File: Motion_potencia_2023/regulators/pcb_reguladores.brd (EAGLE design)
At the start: 200 x 95 mm, 19 parts, among them P1 USB-A1HSW6, X1 5566-25569-2, X3 5566-25569-2

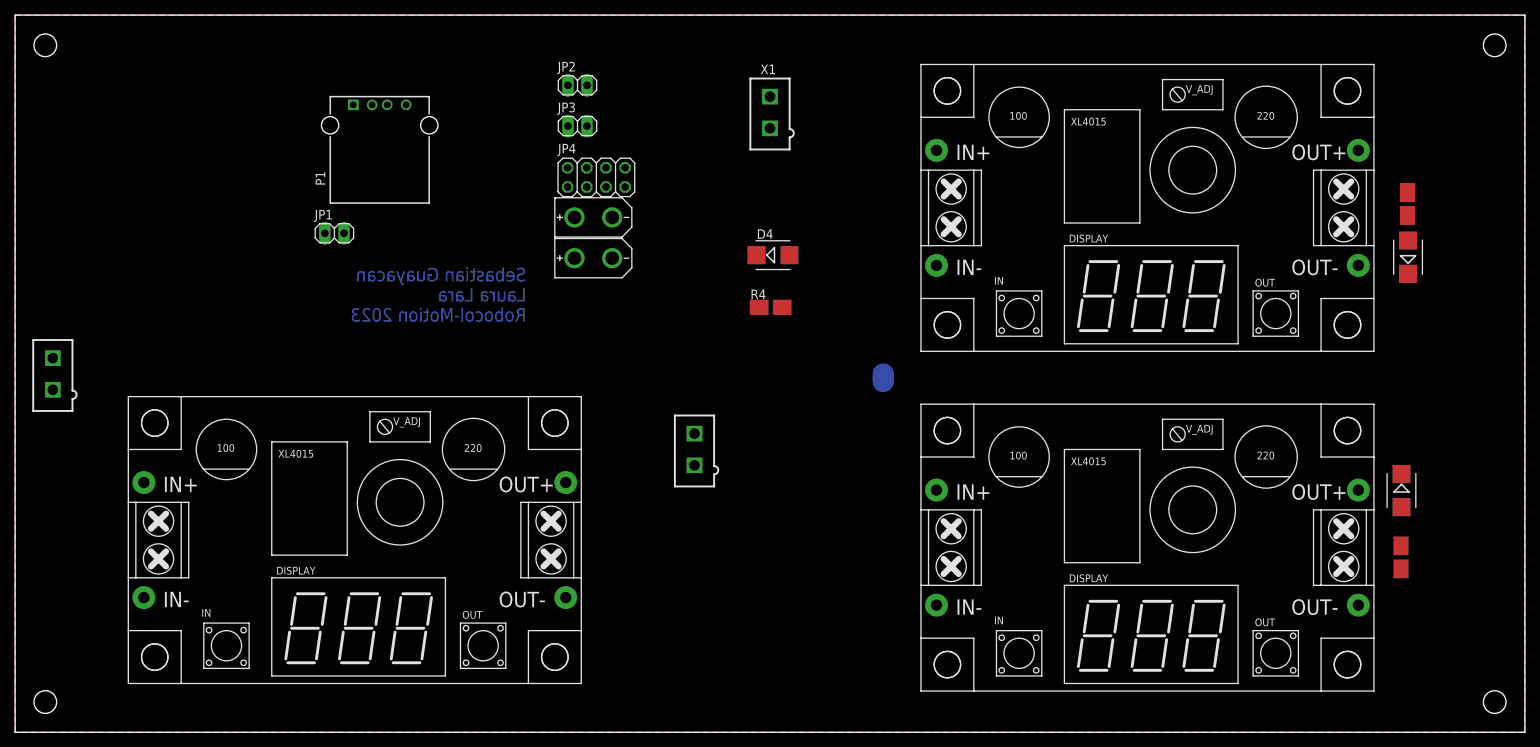
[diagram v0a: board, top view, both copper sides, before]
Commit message: PCBs mandadas a fabricar
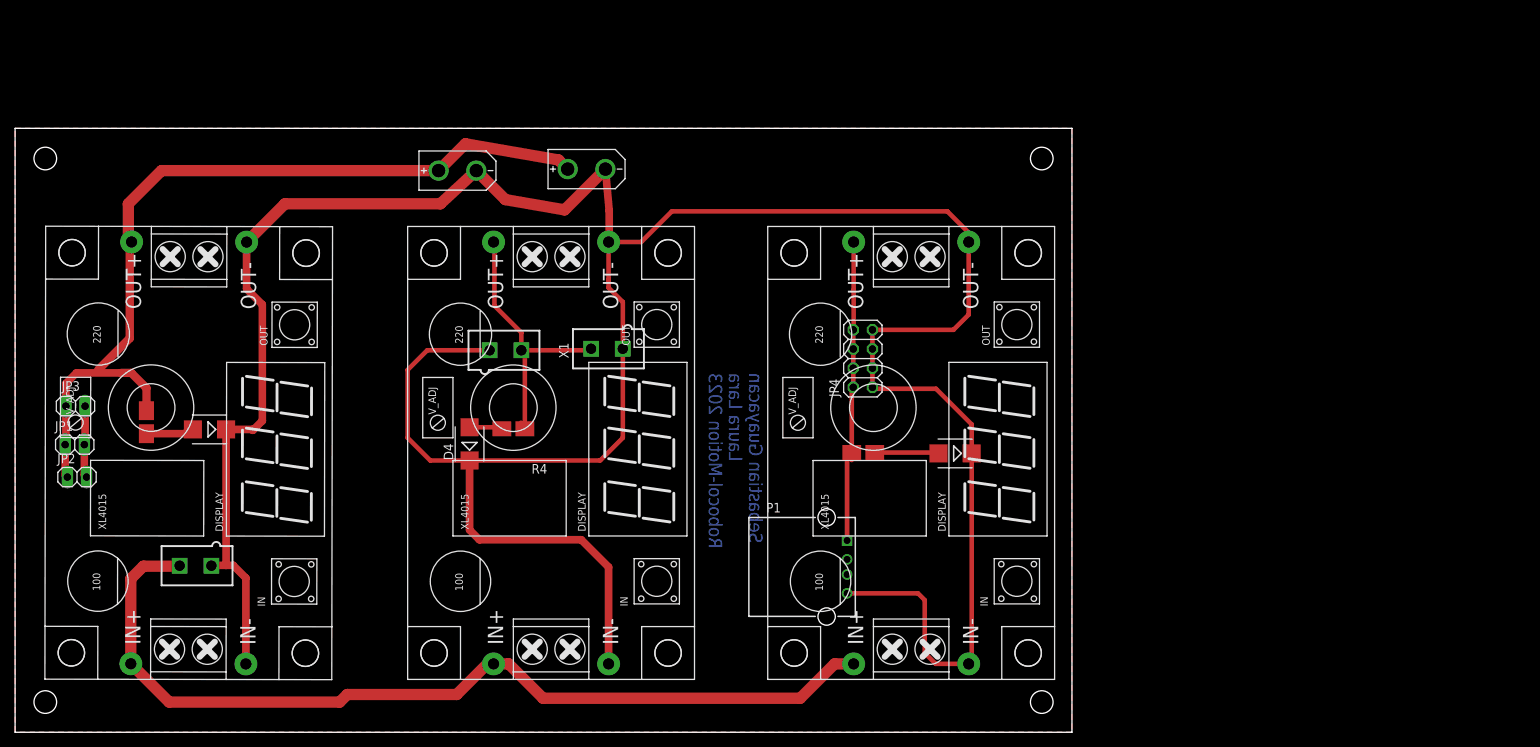
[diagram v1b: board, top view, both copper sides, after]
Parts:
- moved R1 167.2 mm to (17.4, 41.1), turned to 270 degrees
- moved D1 158.1 mm to (25.7, 40.1), turned to 180 degrees
- moved REG12V 127.6 mm to (23.0, 37.0), turned to 89.9 degrees
- moved JP2 84.2 mm to (8.20, 33.8)
- moved R5 79.3 mm to (112.4, 37.1), turned to 0 degrees
- moved P1 77.9 mm to (103.7, 21.9), turned to 270 degrees
- moved JP3 76.1 mm to (8.00, 43.2)
- moved D8 65.4 mm to (124.5, 36.9), turned to 180 degrees
- moved D4 47.3 mm to (60.2, 38.2), turned to 90 degrees
- moved REG5AUX 45.1 mm to (118.7, 37.0), turned to 90 degrees
- moved JP1 44.4 mm to (7.90, 38.1)
- moved JP4 42.7 mm to (112.3, 49.5), turned to 90 degrees
- moved X1 38.0 mm to (78.4, 50.8), turned to 90 degrees
- moved R4 37.7 mm to (66.0, 40.2), turned to 180 degrees
- moved V_IN 31.7 mm to (23.9, 22.1), turned to 90 degrees
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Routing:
- net GND: track 0.00 -> 404.6 mm
- net 24V: track 1.00 -> 122.2 mm
- net OUT12: track 0.00 -> 117.8 mm
- net OUT5AUX: track 0.00 -> 41.0 mm
- net OUT5: track 0.00 -> 36.8 mm
- net N$6: track 0.00 -> 9.57 mm
- net N$20: track 0.00 -> 8.49 mm
- net N$13: track 0.00 -> 6.38 mm
- net N$8: track 0.00 -> 5.07 mm
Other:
- board size 200 x 95 mm -> 140 x 80 mm
